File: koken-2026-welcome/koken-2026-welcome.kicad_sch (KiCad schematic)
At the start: 5 parts, among them J1 USB_C_Receptacle_USB2.0_16P, U1 CH32V003JxMx

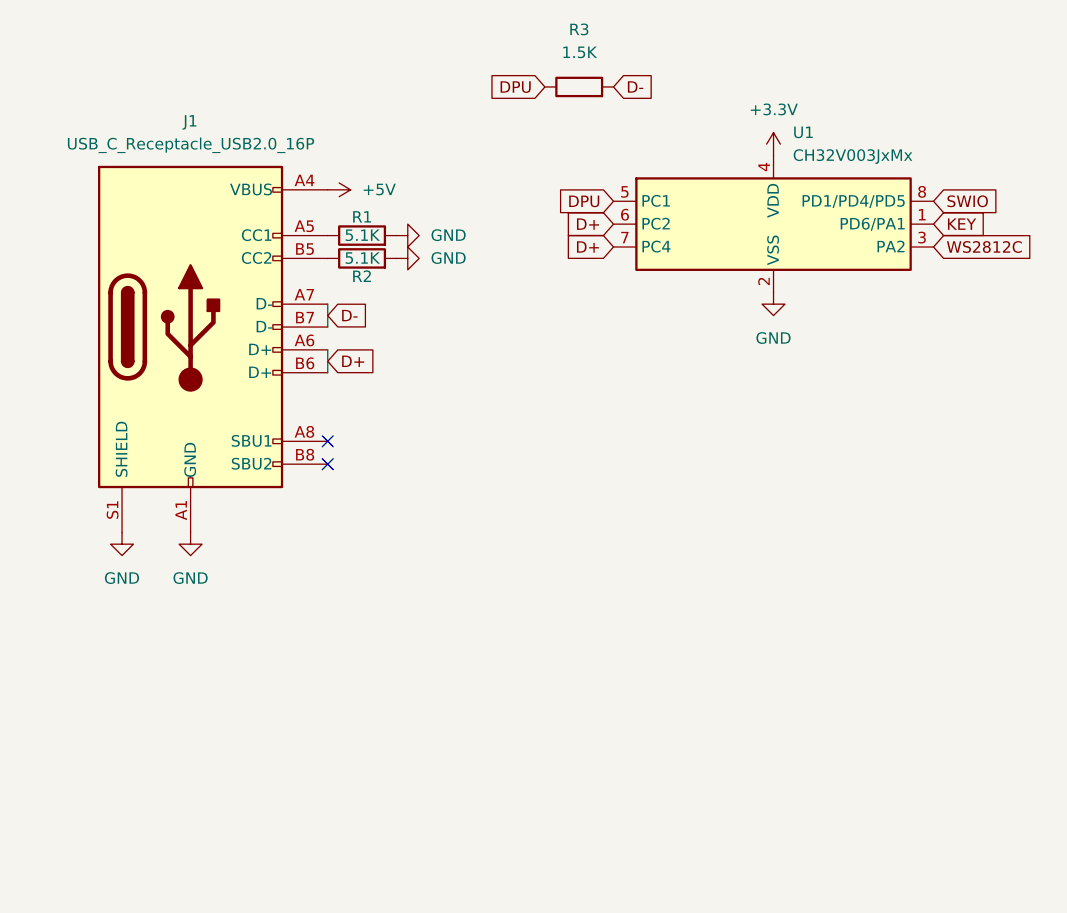
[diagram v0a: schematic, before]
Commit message: add neopixel
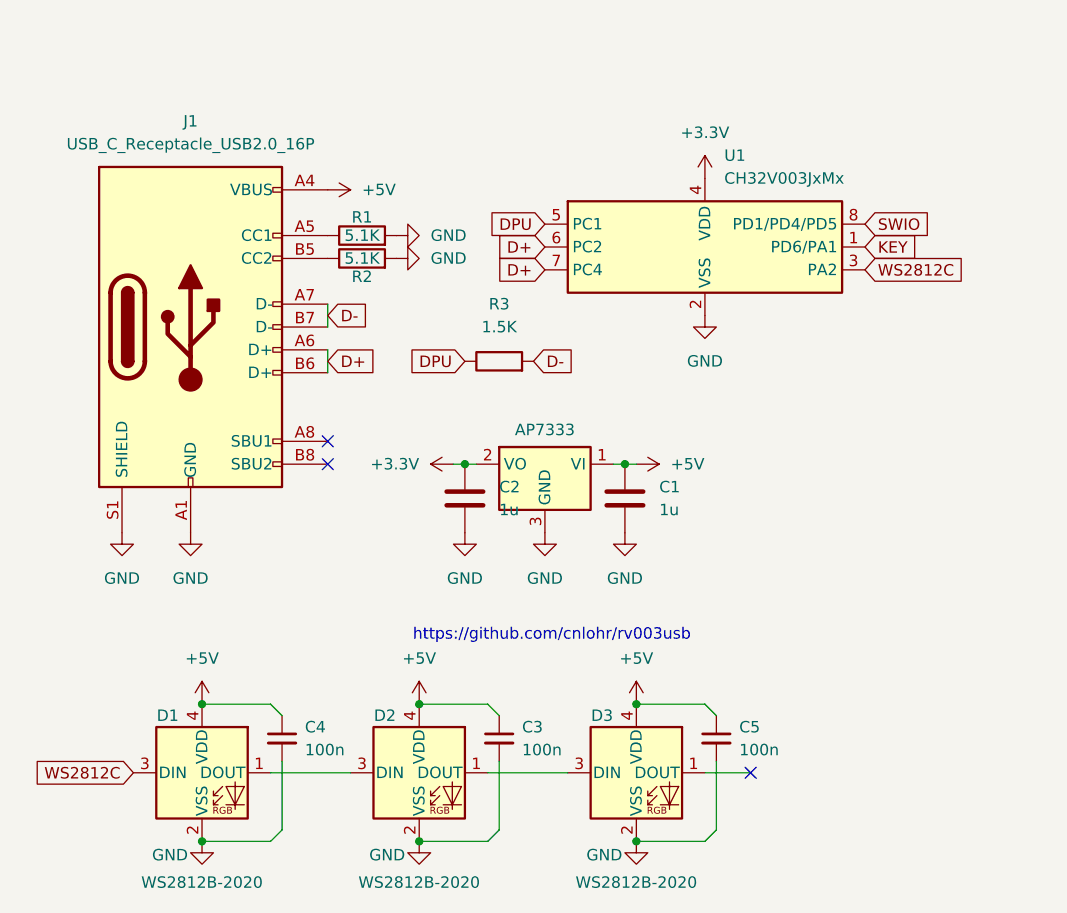
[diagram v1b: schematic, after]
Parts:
- added C1, C2: 1u, symbol Device:C
- added C3, C4, C5: 100n, symbol Device:C_Small
- added D1, D2, D3: WS2812B-2020, LED_SMD:LED_WS2812B-2020_PLCC4_2.0x2.0mm, symbol LED:WS2812B-2020
- added U2: AP7333, Library:AP7333, symbol New_Library:AP7333
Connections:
- net +3.3V: now also C2.1, U2.2 (VO)
- net +5V: now also C1.1, C3.1, C4.1, C5.1, D1.4 (VDD), D2.4 (VDD), D3.4 (VDD), U2.1 (VI)
- net GND: now also C1.2, C2.2, C3.2, C4.2, C5.2, D1.2 (VSS), D2.2 (VSS), D3.2 (VSS), U2.3 (GND)
- net WS2812C: now also D1.3 (DIN)
- new net: D2.1 (DOUT), D3.3 (DIN)
- new net: D1.1 (DOUT), D2.3 (DIN)
- no-connect marks 2 -> 3
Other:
- note added: "https://github.com/cnlohr/rv003usb"
- moved on the sheet: R3, U1
